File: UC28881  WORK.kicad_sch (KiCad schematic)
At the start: 2 parts, among them J1 HV_IN_P, J2 HV_IN_N

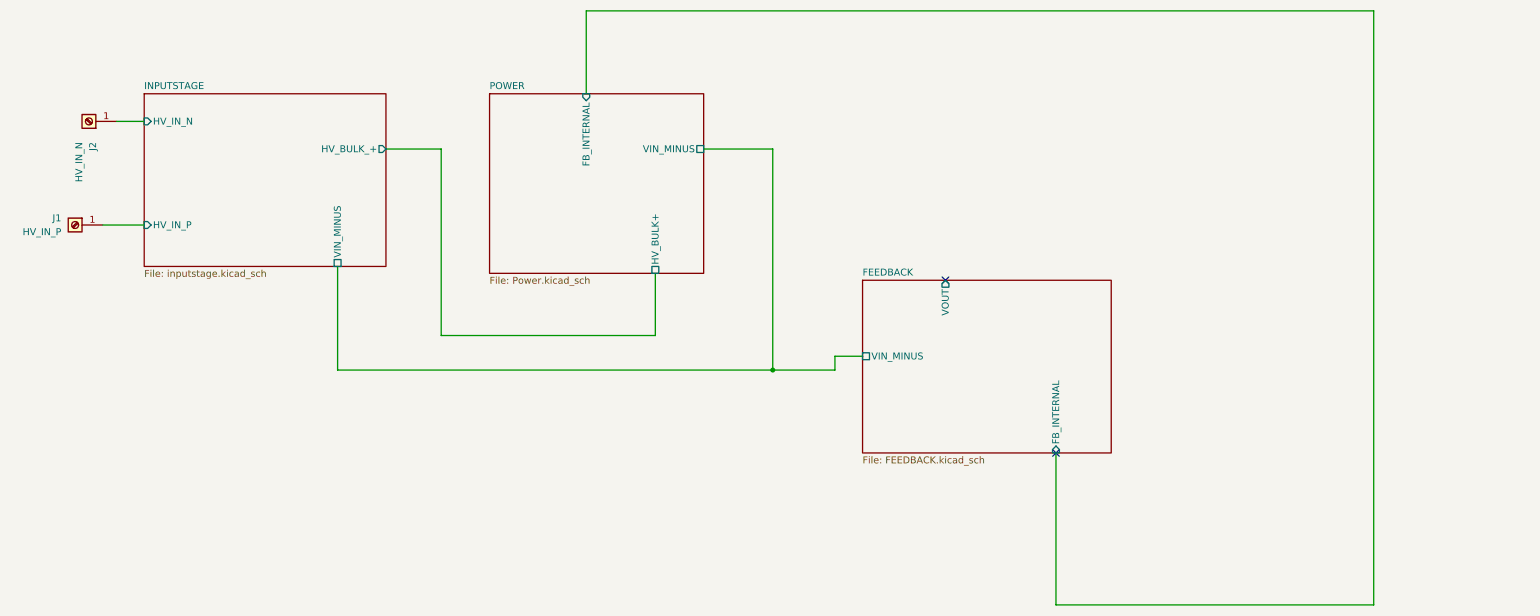
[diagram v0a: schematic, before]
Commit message: Updated KiCad project and schematic files
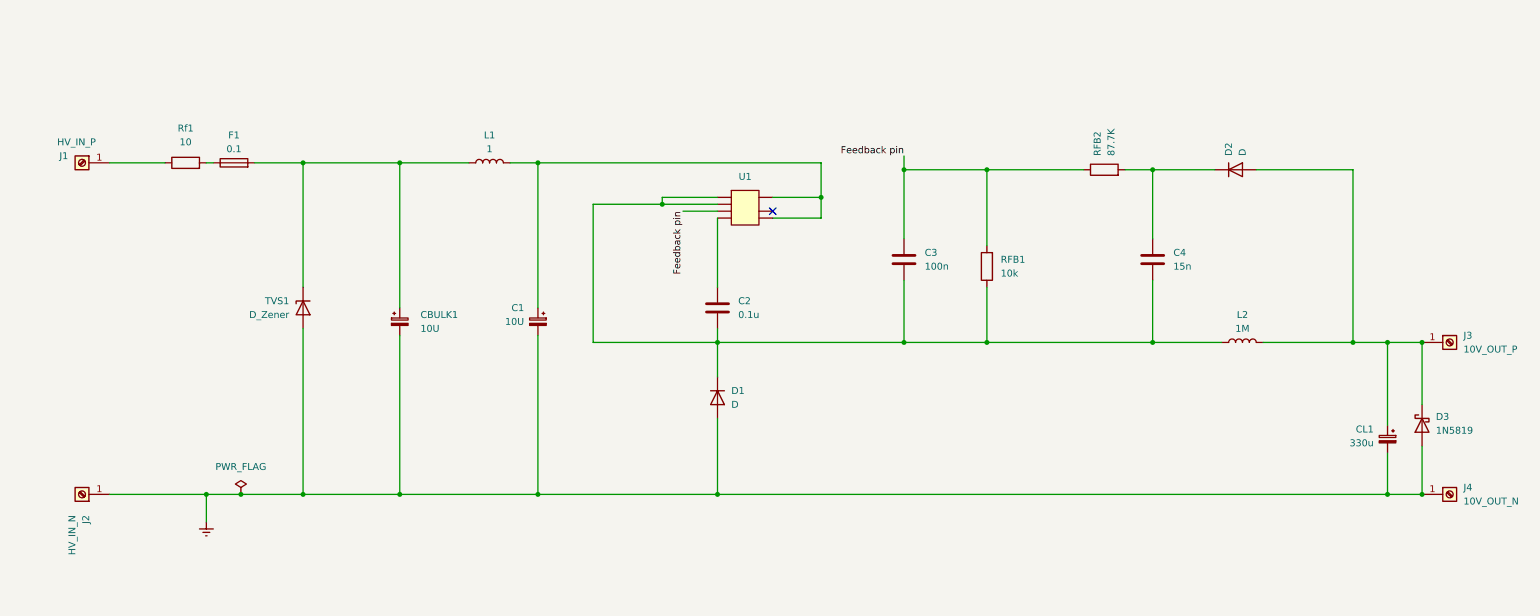
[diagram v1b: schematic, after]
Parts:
- added C1: 10U, Capacitor_THT:CP_Radial_D12.5mm_P7.50mm, symbol Device:C_Polarized_Small
- added C2: 0.1u, Capacitor_THT:C_Rect_L18.0mm_W7.0mm_P15.00mm_FKS3_FKP3, symbol Device:C
- added C3: 100n, Capacitor_THT:C_Rect_L18.0mm_W7.0mm_P15.00mm_FKS3_FKP3, symbol Device:C
- added C4: 15n, Capacitor_THT:C_Rect_L18.0mm_W7.0mm_P15.00mm_FKS3_FKP3, symbol Device:C
- added CBULK1: 10U, Capacitor_THT:CP_Radial_D10.0mm_P5.00mm, symbol Device:C_Polarized_Small
- added CL1: 330u, 350uf:350UF CAP_14102E3_VIS, symbol Device:C_Polarized_Small
- added D1, D2: D, symbol Device:D
- added D3: 1N5819, Diode_THT:D_DO-41_SOD81_P10.16mm_Horizontal, symbol Diode:1N5819
- added F1: 0.1, 100nf:100NF CAPC1005X55N, symbol Device:Fuse
- added J3: 10V_OUT_P, symbol Connector:Screw_Terminal_01x01
- added J4: 10V_OUT_N, symbol Connector:Screw_Terminal_01x01
- added L1: 1, Inductor_SMD:L_7.3x7.3_H3.5, symbol Device:L
- added L2: 1M, Inductor_SMD:L_12x12mm_H8mm, symbol Device:L
- added RFB1: 10k, 10k resistor:RESC2012X65N, symbol Device:R
- added RFB2: 87.7K, 121k resistor:121K RES_ERJ8ENF1213V, symbol Device:R
- added Rf1: 10, Resistor_THT:R_Axial_DIN0922_L20.0mm_D9.0mm_P30.48mm_Horizontal, symbol Device:R
- added TVS1: D_Zener, symbol Device:D_Zener
- added U1: UCC28881, UCC2881:TI_SOIC-8_D_UCC28881_1.27mm, symbol New_Library for UCC28881:UCC28881
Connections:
- net INPUTSTAGE/HV_IN_N renamed Earth
- net Earth: now also C1.2, CBULK1.2, CL1.2, D1.2 (A), D3.2 (A), J4.1 (Pin_1), TVS1.2 (A)
- net INPUTSTAGE/HV_IN_P: no longer names the net of J1.1 (Pin_1)
- net INPUTSTAGE/HV_IN_P: now also Rf1.1
- new net: C1.1, L1.2, U1.5 (HVIN), U1.8 (DRAIN)
- new net: C2.2, C3.2, C4.2, D1.1 (K), L2.1, RFB1.1, U1.1 (GND), U1.2 (GND)
- new net: F1.1, Rf1.2
- new net: CBULK1.1, F1.2, L1.1, TVS1.1 (K)
- new net: CL1.1, D2.2 (A), D3.1 (K), J3.1 (Pin_1), L2.2
- new net: C4.1, D2.1 (K), RFB2.2
- new net: C2.1, U1.4 (VDD)
- new net Feedback pin: C3.1, RFB1.2, RFB2.1, U1.3 (FB)
- no-connect marks 2 -> 1
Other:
- removed sheet FEEDBACK
- removed sheet INPUTSTAGE
- removed sheet POWER
- moved on the sheet: J1
